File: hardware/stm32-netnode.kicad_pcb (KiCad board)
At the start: 4 copper layers, 60 x 60 mm, 96 parts, among them J1 USB4110-GF-A, J2 J0011D01BNL, J4 Breakout, SW1 7914J-1-000E, SW2 7914J-1-000E, U1 STM32F407VETx, U2 W25Q25PWSSIQ, U3 LAN8720A, U4 BME688, U5 CP2102N-A02-GQFN20R, U6 AP2112K-3.3, U7 USBLC6-2P6, Y1 8MHz, Y2 ABM3B-25.000MHZ-B2-T

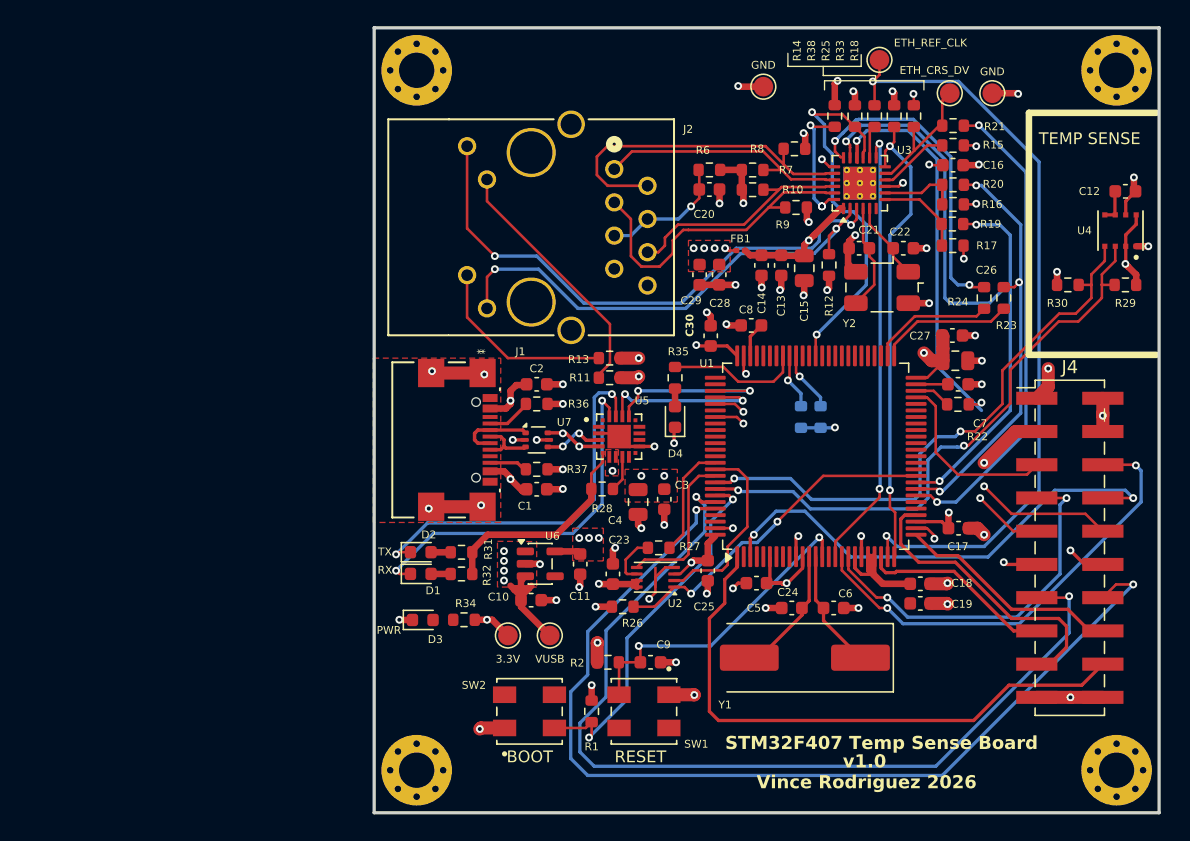
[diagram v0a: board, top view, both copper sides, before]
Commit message: Radd rev 2.0
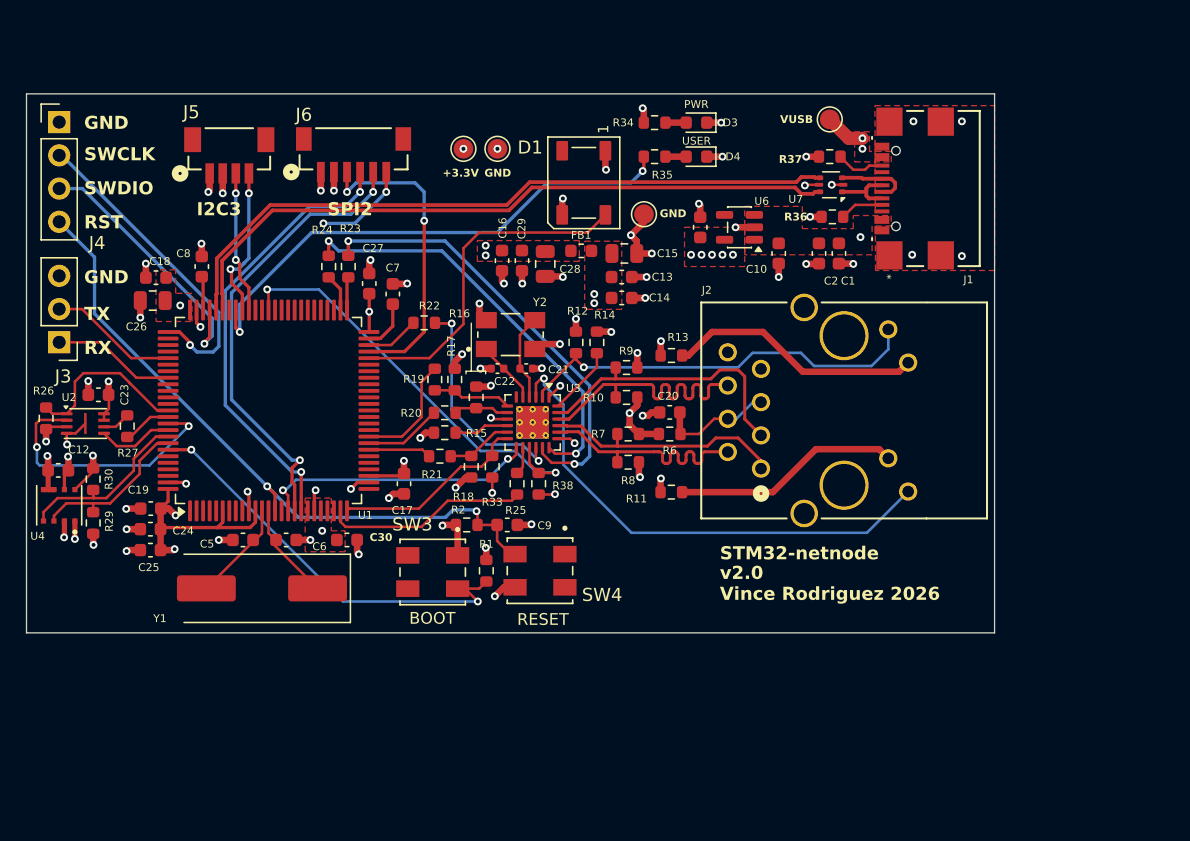
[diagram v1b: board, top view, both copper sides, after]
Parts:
- removed C3: 0.1u, Capacitor_SMD:C_0603_1608Metric
- removed C4: 4.7u, Capacitor_SMD:C_0805_2012Metric
- removed D2: LED, LED_SMD:LED_0603_1608Metric
- removed ETH_CRS_DV, ETH_REF_CLK: TestPoint, TestPoint:TestPoint_Pad_D1.5mm
- removed H1, H2, H3, H4: MountingHole_Pad, MountingHole:MountingHole_2.7mm_M2.5_Pad_Via
- removed R28: 1k, Resistor_SMD:R_0603_1608Metric
- removed R3, R4: 4.7k, Resistor_SMD:R_0603_1608Metric
- removed R31, R32: 220, Resistor_SMD:R_0603_1608Metric
- removed SW1, SW2: 7914J-1-000E, footprints:SW_7914J-1-000E
- removed U5: CP2102N-A02-GQFN20R, footprints:SILABS_CP2102N-A02-GQFN20R
- added J3: UART5, Connector_PinHeader_2.54mm:PinHeader_1x03_P2.54mm_Vertical, F.Cu at (93.5, 94.8)
- added J5: I2C, footprints:CONN4_BM04B-SRSS_JST, F.Cu at (106.5, 80.0)
- added J6: SPI2, footprints:CONN_BM06B-SRSS-TB_JST, F.Cu at (116.0, 80.0)
- added SW3: BOOT0, footprints:SW_7914J-1-000E, F.Cu at (122.0, 112.3)
- added SW4: NRST, footprints:SW_7914J-1-000E, F.Cu at (130.2, 112.2)
- C1: value 10u -> 100nF
- C2: value 10u -> 4.7u
- C21, C22: value 27pF -> 12pF; footprint Capacitor_SMD:C_0603_1608Metric -> Capacitor_SMD:C_0402_1005Metric
- C28: value 10u -> 4.7u; footprint Capacitor_SMD:C_0603_1608Metric -> Capacitor_SMD:C_0805_2012Metric
- D1: value LED -> WS2812B; footprint LED_SMD:LED_0603_1608Metric -> LED_SMD:LED_WS2812B_PLCC4_5.0x5.0mm_P3.2mm
- FB1: footprint Inductor_SMD:L_0201_0603Metric -> Inductor_SMD:L_0603_1608Metric
- J4: value Breakout -> SWD; footprint Connector_PinHeader_2.54mm:PinHeader_2x10_P2.54mm_Vertical_SMD -> Connector_PinHeader_2.54mm:PinHeader_1x04_P2.54mm_Vertical
- R27: value 10k -> 0
- U2: value W25Q25PWSSIQ -> W25Q80DVUXIE TR
- Y2: value ABM3B-25.000MHZ-B2-T -> ECS-250-8-30B-CKM; footprint Crystal:Crystal_SMD_Abracon_ABM3B-4Pin_5.0x3.2mm -> footprints:XTAL_ECS-250-8-30B-CKM
- moved C12 84.3 mm to (93.4, 104.6)
- moved J4 83.8 mm to (93.5, 78.0)
- moved U4 83.8 mm to (93.5, 107.2)
- moved R29 81.0 mm to (96.1, 108.6), turned to 90 degrees
- moved R30 76.0 mm to (96.1, 105.2), turned to -90 degrees
- moved C18 62.9 mm to (100.9, 89.8), turned to 180 degrees
- moved C26 61.5 mm to (100.7, 91.6), turned to 180 degrees
- moved C19 59.3 mm to (100.5, 107.5), turned to 180 degrees
- moved R23 50.2 mm to (115.6, 89.0)
- moved R24 50.2 mm to (114.1, 89.0)
- moved R21 46.7 mm to (122.6, 103.5), turned to 0 degrees
- moved C24 46.5 mm to (100.5, 109.1)
- moved R26 46.4 mm to (92.5, 100.6), turned to 90 degrees
- moved U2 45.1 mm to (95.5, 101.0), turned to 0 degrees
- moved TP2 44.9 mm to (152.4, 77.8)
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- renumbered 3.3V to TP1, VUSB to TP2, GND to TP3, GND to TP4
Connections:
- C16 pad 1: VDDIO -> +3.3V
- C9 pad 1: /NRST -> NRST
- D1 pad 1: Net-(D1-K) -> +3.3V
- D1 pad 2: Net-(D1-A) -> unconnected-(D1-DOUT-Pad2)
- J2 pad 8: unconnected-(J2-GND-Pad8) -> GND
- J4 pad 1: +3.3V -> GND
- J4 pad 2: GND -> SWCLK
- J4 pad 3: VUSB -> SWDIO
- J4 pad 4: GND -> NRST
- R15 pad 1: VDDIO -> +3.3V
- R16 pad 1: VDDIO -> +3.3V
- R17 pad 1: VDDIO -> +3.3V
- R18 pad 1: VDDIO -> +3.3V
- R2 pad 2: /NRST -> NRST
- R26 pad 2: /FLASH_CE -> FLASH_CE
- U1 pad 1: GPIO1 -> unconnected-(U1-PE2-Pad1)
- U1 pad 14: /NRST -> NRST
- U1 pad 23: ADC1_IN0 -> unconnected-(U1-PA0-Pad23)
- U1 pad 26: ADC1_IN3 -> unconnected-(U1-PA3-Pad26)
- U1 pad 29: DAC1_OUT -> unconnected-(U1-PA4-Pad29)
- U1 pad 3: SPI2_CS -> unconnected-(U1-PE4-Pad3)
- U1 pad 35: /FLASH_CE -> unconnected-(U1-PB0-Pad35)
- U1 pad 46: unconnected-(U1-PE15-Pad46) -> NEOPIX
- U1 pad 70: unconnected-(U1-PA11-Pad70) -> USB_D-
- U1 pad 71: unconnected-(U1-PA12-Pad71) -> USB_D+
- U1 pad 72: unconnected-(U1-PA13-Pad72) -> SWDIO
- U1 pad 76: unconnected-(U1-PA14-Pad76) -> SWCLK
- U1 pad 78: UART4_TX -> unconnected-(U1-PC10-Pad78)
- U1 pad 79: UART4_RX -> unconnected-(U1-PC11-Pad79)
- U1 pad 82: UART5_RX -> unconnected-(U1-PD1-Pad82)
- U1 pad 83: unconnected-(U1-PD2-Pad83) -> UART5_RX
- U1 pad 88: unconnected-(U1-PD7-Pad88) -> FLASH_CE
- U1 pad 95: PWM_TIM4_CH3 -> unconnected-(U1-PB8-Pad95)
- U1 pad 96: PWM_TIM4_CH4 -> unconnected-(U1-PB9-Pad96)
- U2 pad 1: /FLASH_CE -> FLASH_CE
- U3 pad 9: VDDIO -> +3.3V
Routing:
- net PWM_TIM4_CH4: track 76.8 -> 0.00 mm, vias 2 -> 0
- net PWM_TIM4_CH3: track 72.7 -> 0.00 mm, vias 2 -> 0
- net NRST: track 0.00 -> 51.8 mm, vias 0 -> 2
- net USB_D+: track 4.56 -> 52.7 mm, vias 2 -> 0
- net USB_D-: track 4.33 -> 52.1 mm, vias 2 -> 0
- net GPIO1: track 44.9 -> 0.00 mm
- net /ETH_REF_CLK_MCU: track 59.6 -> 15.6 mm, vias 2 -> 0
- net SDA: track 45.4 -> 12.5 mm, vias 2 -> 0
- net /ETH_CRS_DV: track 36.9 -> 4.81 mm, vias 2 -> 0
- net SCL: track 44.6 -> 13.8 mm, vias 2 -> 0
- net SPI2_CS: track 37.8 -> 7.32 mm
- net Net-(U1-PA9): track 10.3 -> 40.1 mm, vias 0 -> 2
- net Net-(D1-K): track 29.2 -> 0.00 mm, vias 2 -> 0
- net Net-(D2-K): track 28.4 -> 0.00 mm, vias 2 -> 0
- net UART5_RX: track 37.8 -> 9.45 mm, vias 2 -> 0
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- added copper zone on F.Cu, net VDDA
- added copper zone on In2.Cu, net VDDA
- removed copper zone on In2.Cu, net VDDIO
- removed copper zone on In2.Cu, net VUSB
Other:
- board size 60 x 60 mm -> 74 x 41.2 mm
- board text added: "+3.3V"
- board text added: "GND"
- board text added: "I2C3"
- board text added: "RST"
- board text added: "SPI2"
- board text added: "STM32-netnode"
- board text added: "SWCLK"
- board text added: "SWDIO"
- board text added: "USER"
- board text added: "VUSB"
- board text added: "v2.0"
- board text removed: "STM32F407 Temp Sense Board"
- board text removed: "TEMP SENSE"
- board text removed: "v1.0"
